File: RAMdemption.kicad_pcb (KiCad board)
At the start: 4 copper layers, 99 x 53.5 mm, 41 parts, among them J1 Conn_RAM_Expansion, U1 TC518512FTL-70, U10 TC518512FTL-70, U11 TC518512FTL-70, U12 TC518512FTL-70, U13 TC518512FTL-70, U14 TC518512FTL-70, U15 TC518512FTL-70, U16 TC518512FTL-70, U17 TC518512FTL-70, U18 TC518512FTL-70, U19 TC518512FTL-70, U2 TC518512FTL-70, U20 TC518512FTL-70, U3 TC518512FTL-70, U4 TC518512FTL-70, U5 TC518512FTL-70, U6 TC518512FTL-70, U7 TC518512FTL-70, U8 TC518512FTL-70, U9 TC518512FTL-70

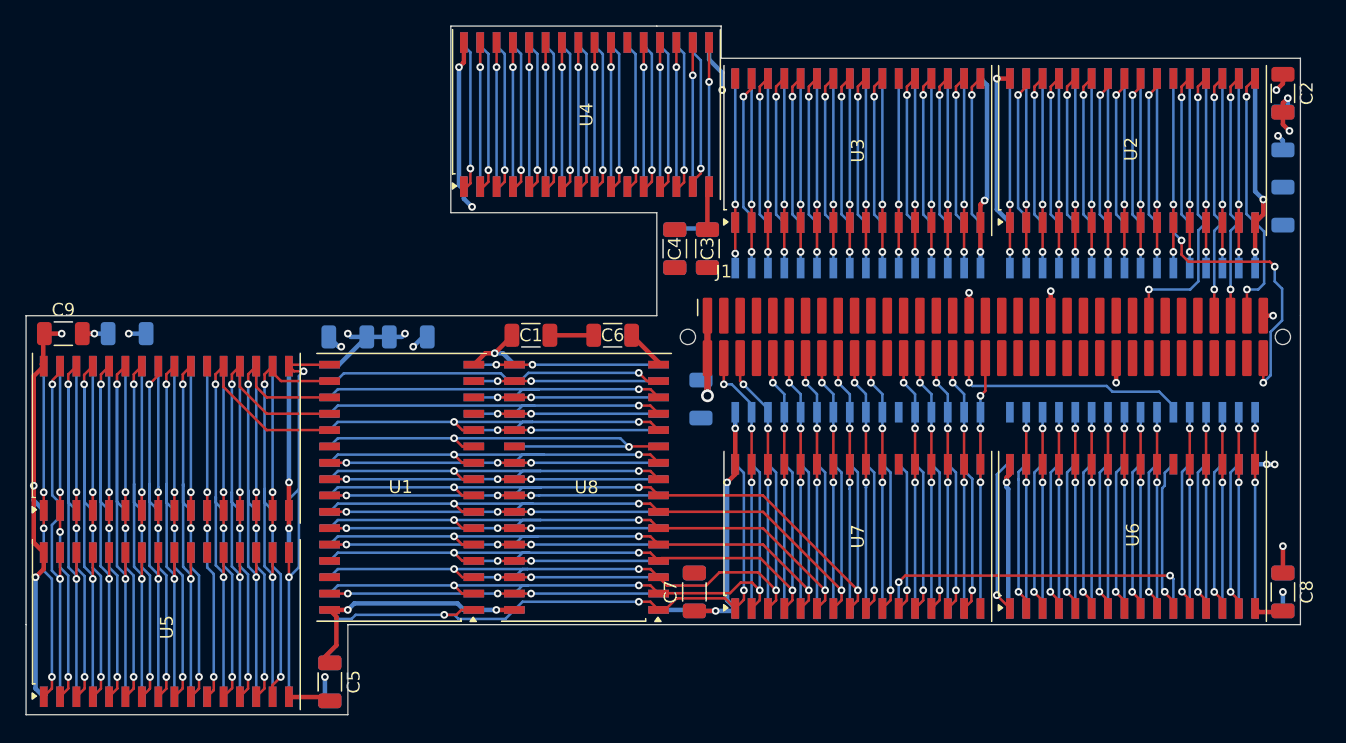
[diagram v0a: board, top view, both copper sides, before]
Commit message: shuffle around files
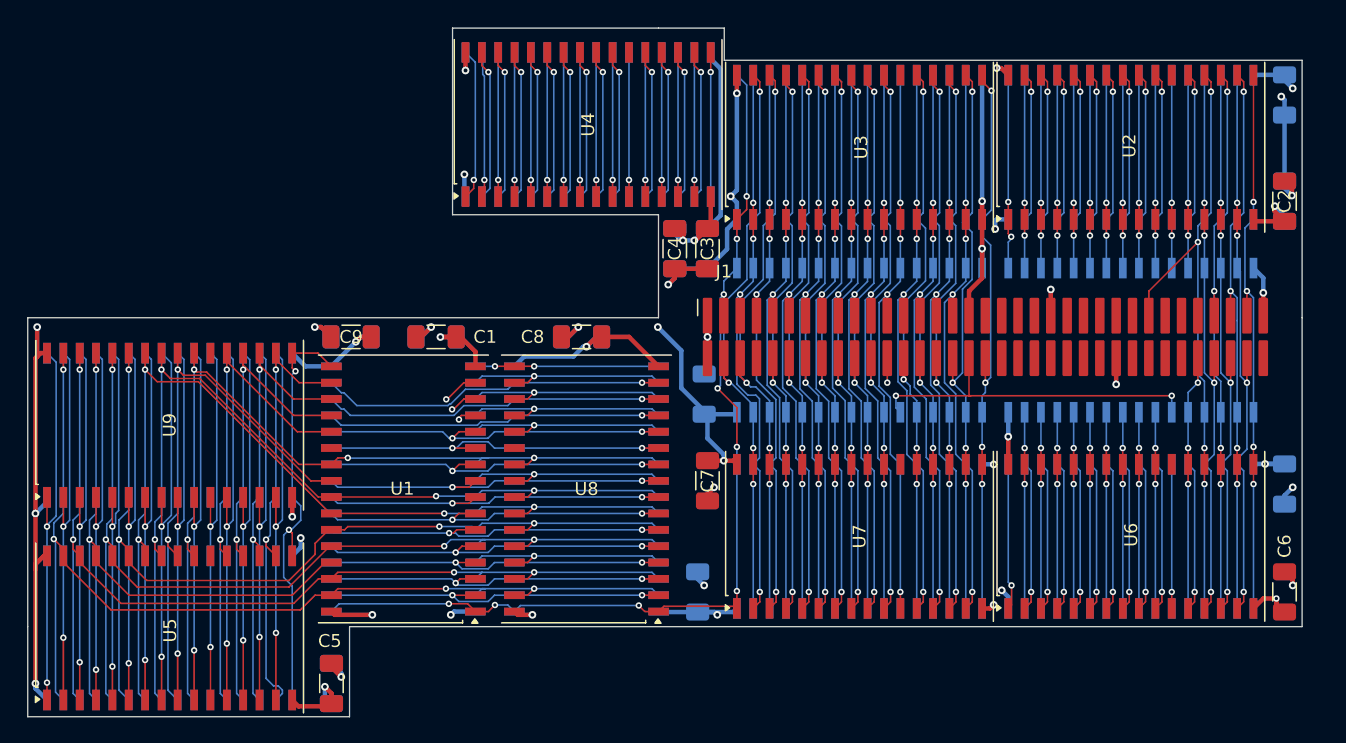
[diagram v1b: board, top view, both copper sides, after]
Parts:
- C1, C10, C11, C12, C13, C14, C15, C16, C17, C18, C19, C2, C20, C3, C4, C5, C6, C7, C8, C9: footprint Capacitor_SMD:C_1206_3216Metric -> Capacitor_SMD:C_1206_3216Metric_Pad1.33x1.80mm_HandSolder
- J1: footprint RAMdemption:TE_5-104652-7 -> RAMdemption:TE_5-104652-7_NoHoles
- moved C8 58.0 mm to (154.2, 103.5), turned to 0 degrees
- moved C6 55.9 mm to (208.8, 123.3), turned to -90 degrees
- moved U20 31.7 mm to (154.7, 87.0), turned to -90 degrees
- moved U12 29.1 mm to (154.5, 115.3), turned to 0 degrees
- moved C9 22.4 mm to (136.2, 103.5)
- moved C17 17.4 mm to (136.2, 103.5), turned to 0 degrees
- moved U16 14.2 mm to (140.3, 115.3)
- moved C14 13.5 mm to (154.2, 103.5), turned to 0 degrees
- moved C7 8.70 mm to (163.9, 114.7), turned to -90 degrees
- moved C2 8.38 mm to (208.8, 93.0)
- moved C11 8.38 mm to (208.8, 114.9), turned to 90 degrees
- moved C1 7.37 mm to (142.9, 103.5), turned to 0 degrees
- moved C18 6.86 mm to (142.9, 103.5)
- moved C19 2.80 mm to (208.8, 84.7)
- moved U17 1.05 mm to (122.2, 110.4)
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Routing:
- net +5V: track 128.8 -> 432.9 mm, vias 20 -> 28
- net /RAM Bank 1/A18: track 127.3 -> 181.0 mm, vias 12 -> 15
- net /RAM Bank 1/A16: track 129.4 -> 176.9 mm
- net /RAM Bank 1/A3: track 121.1 -> 167.8 mm
- net /RAM Bank 1/A2: track 121.3 -> 166.9 mm
- net /RAM Bank 1/A0: track 120.4 -> 165.9 mm
- net /RAM Bank 1/A14: track 130.4 -> 173.3 mm
- net /RAM Bank 1/A17: track 122.8 -> 163.8 mm
- net /RAM Bank 1/A15: track 124.6 -> 165.5 mm, vias 13 -> 12
- net /RAM Bank 1/A12: track 131.7 -> 172.0 mm
- net /RAM Bank 1/A1: track 127.8 -> 165.8 mm
- net /RAM Bank 1/A7: track 134.0 -> 171.2 mm
- net /RAM Bank 1/A6: track 136.0 -> 170.3 mm
- net /RAM Bank 1/A9: track 125.8 -> 159.0 mm, vias 13 -> 12
- net /RAM Bank 1/A5: track 137.2 -> 169.5 mm
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- removed copper zone on In2.Cu, net +5V
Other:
- outline, holes or cut-outs redrawn
